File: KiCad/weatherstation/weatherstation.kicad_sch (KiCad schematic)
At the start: 6 parts, among them U1 ESP32_NODEMCU, U2 AM2302, U3 AM2302

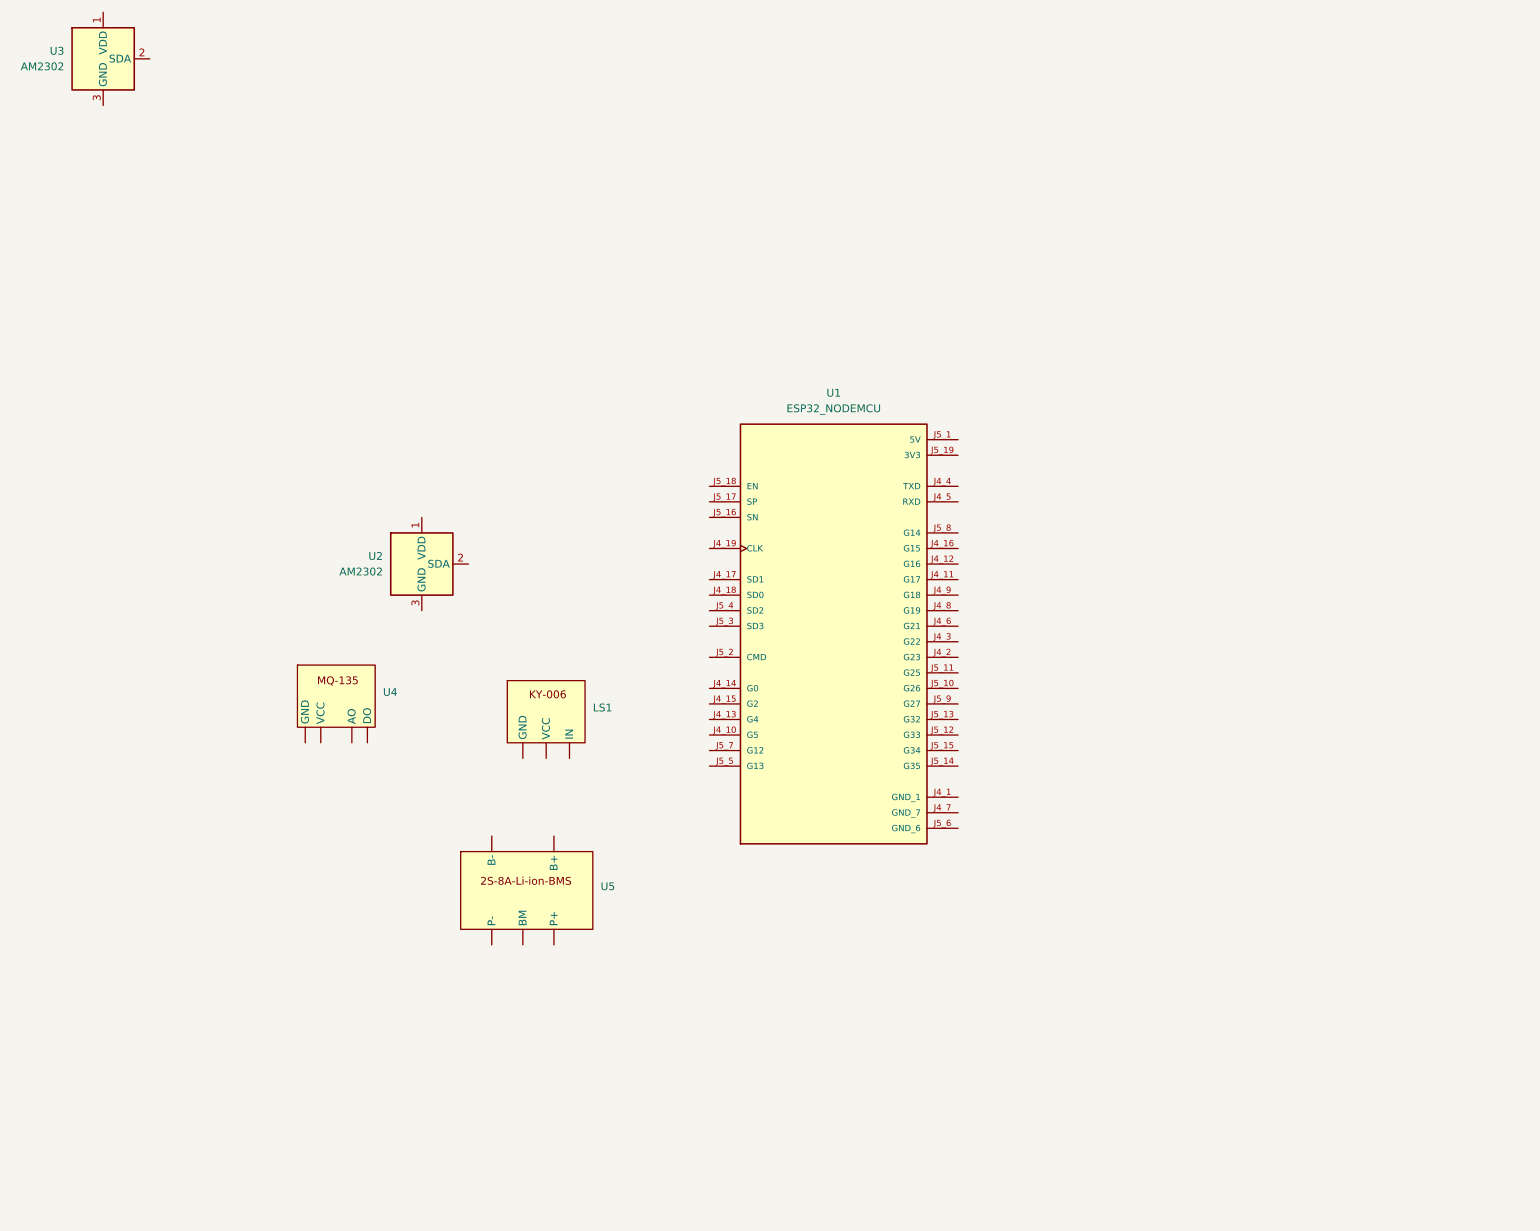
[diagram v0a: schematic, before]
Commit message: dighdfiug
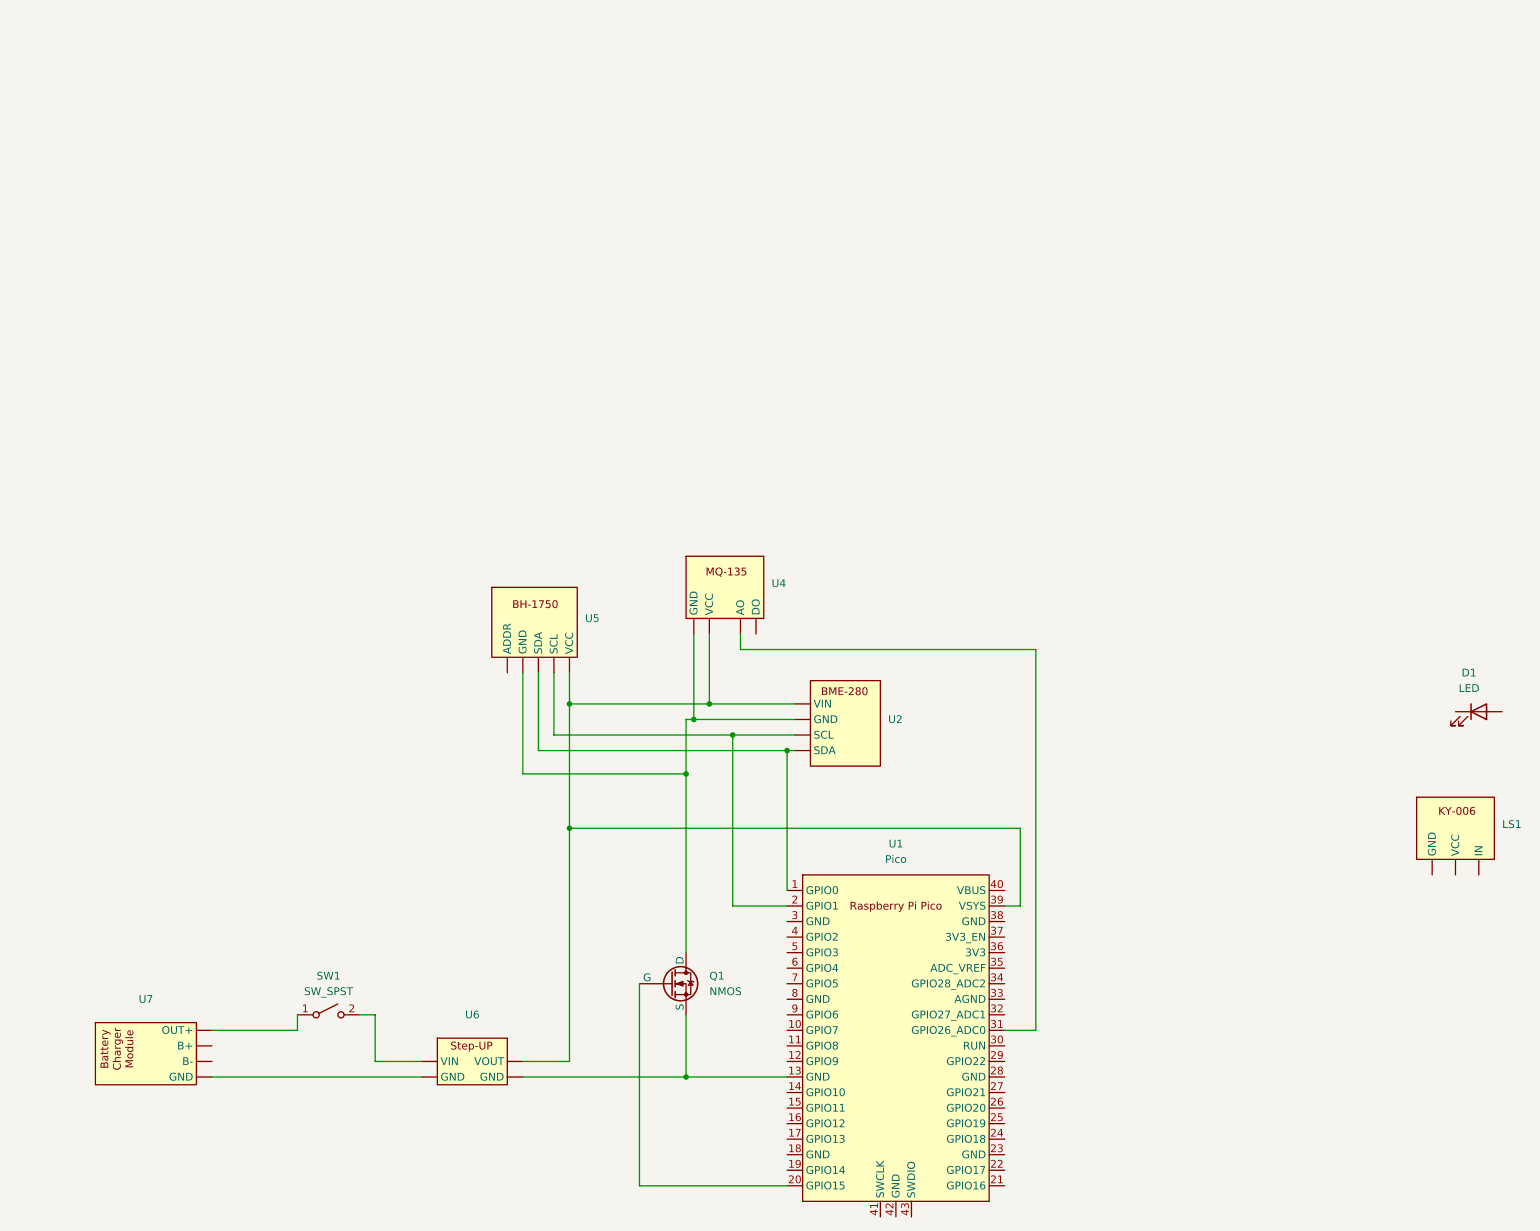
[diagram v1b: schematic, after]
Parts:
- removed U1: ESP32_NODEMCU, ESP32_NODEMCU:MODULE_ESP32_NODEMCU, symbol weatherstation:ESP32_NODEMCU
- removed U2, U3: AM2302, Sensor:ASAIR_AM2302_P2.54mm_Vertical, symbol Sensor:AM2302
- removed U5: ~, symbol weatherstation:2S-8A-Li-ion-Lithium-18650-BMS{lt}
- added D1: LED, symbol Device:LED
- added Q1: NMOS, symbol Simulation_SPICE:NMOS
- added SW1: SW_SPST, symbol Switch:SW_SPST
- added U1: Pico, RPi_Pico:RPi_Pico_SMD_TH, symbol MCU_RaspberryPi_and_Boards:Pico
- added U2: ~, symbol weatherstation:bme280
- added U5: ~, symbol weatherstation:bh1750
- added U6: ~, symbol weatherstation:Step-up
- added U7: ~, symbol weatherstation:Battery-Charger-Module
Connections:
- net at U4. (VCC): now also Q1.1 (D), U2. (VIN), U5. (VCC)
- new net: U1.31 (GPIO26_ADC0), U4. (VCC)
- new net: U1.39 (VSYS), U2. (VIN), U4. (VCC), U5. (VCC), U6. (VOUT)
- new net: U1.1 (GPIO0), U2. (VIN), U5. (VCC)
- new net: Q1.3 (S), U1.13 (GND), U6. (VOUT)
- new net: U1.2 (GPIO1), U2. (VIN), U5. (VCC)
- new net: Q1.2 (G), U1.20 (GPIO15)
- new net: SW1.1 (A), U7. (OUT+)
- new net: U6. (VOUT), U7. (OUT+)
- new net: SW1.2 (B), U6. (VOUT)
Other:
- moved on the sheet: LS1, U4
